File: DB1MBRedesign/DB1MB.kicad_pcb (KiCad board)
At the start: 4 copper layers, 124.5 x 69.2 mm, 160 parts, among them J7 Conn_01x04_Socket, J8 DIN41612_03x10_ABC, J9 DIN41612_03x10_ABC, Q1 Q_Photo_NPN_CBE, Q2 Q_Photo_NPN_CBE, Q3 BSS84, Q4 IRF7313, Q5 BC807-40W, Q6 BC846, U1 MC68331, U11 74LS08, U2 ATmega48V-10A, U3 CY62157, U4 74LS573, U5 74LS245, U6 74LS573, U7 74LS573, U8 74LS245, U9 74LS20, Y1 32.768k

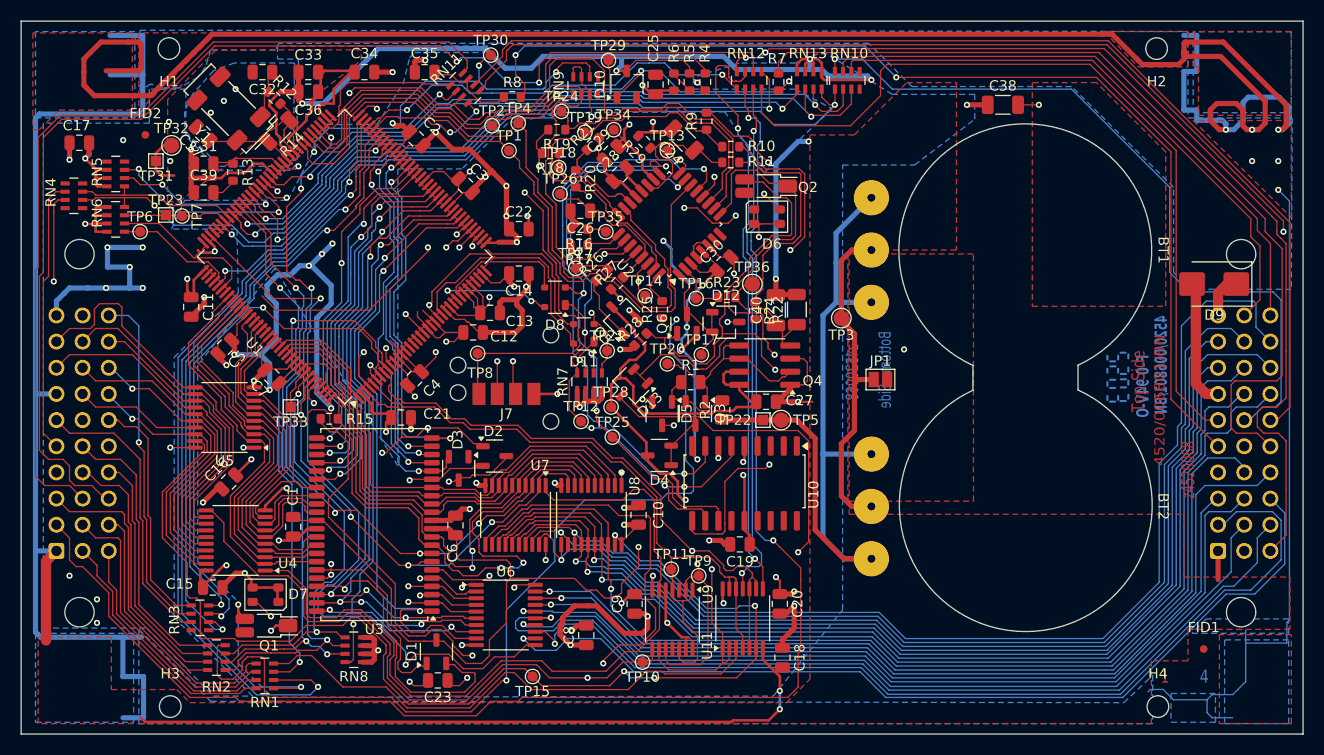
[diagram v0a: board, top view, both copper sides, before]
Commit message: rtc
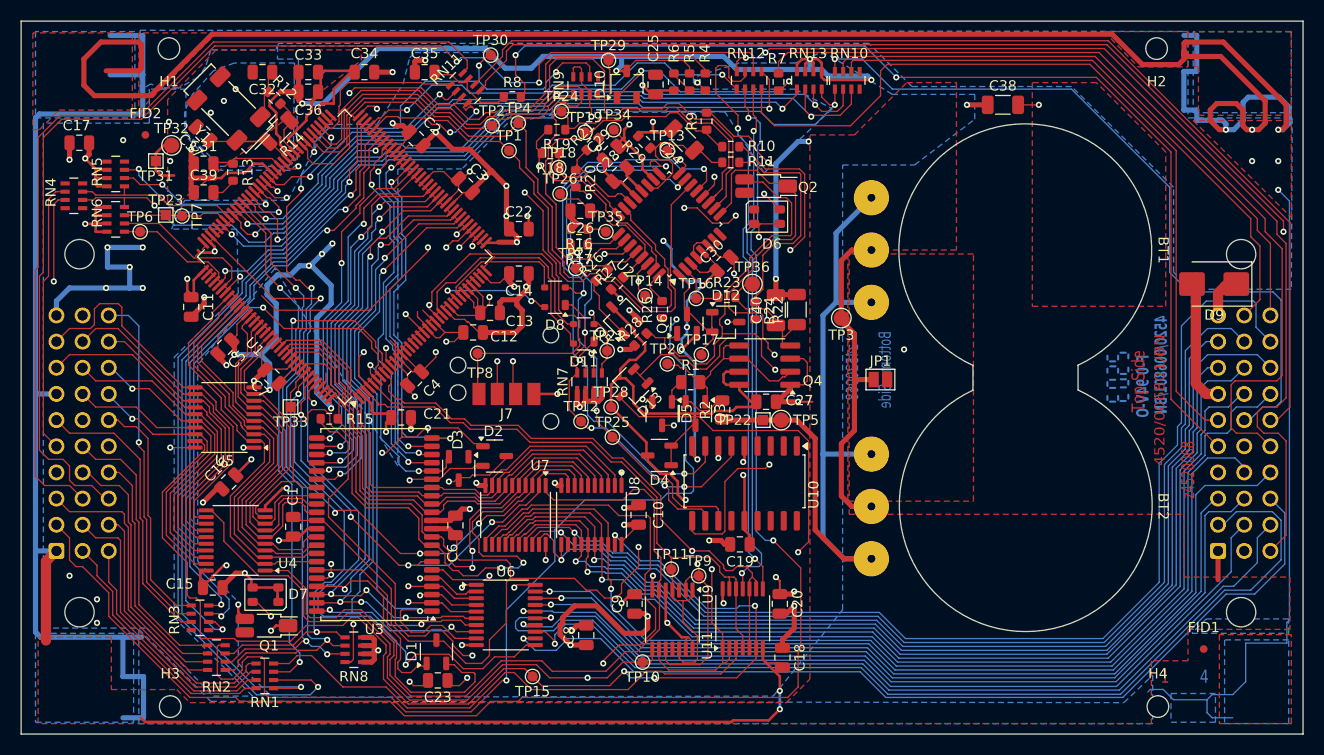
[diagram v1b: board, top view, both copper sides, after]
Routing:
- net A0: track 6.21 -> 56.2 mm, vias 1 -> 2
- net A1: track 8.37 -> 45.5 mm
- net A3: track 10.2 -> 46.6 mm
- net A2: track 8.06 -> 43.4 mm
- net GND: track 710.2 -> 726.3 mm
- net VDD: track 420.1 -> 427.2 mm
- net Net-(U1-EXTAL): track 7.98 -> 12.4 mm
- net PQS3: track 13.5 -> 14.9 mm
- net PD7: track 26.6 -> 28.0 mm
- net Net-(U2-ADC6): track 14.1 -> 15.2 mm
- net Net-(Q4B-G): track 12.3 -> 13.4 mm
- net Net-(U2-ADC7): track 8.21 -> 9.29 mm
- net Net-(Q3-G): track 20.1 -> 21.0 mm
- net PD1: track 37.4 -> 38.3 mm
- net PD3: track 12.0 -> 12.9 mm
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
